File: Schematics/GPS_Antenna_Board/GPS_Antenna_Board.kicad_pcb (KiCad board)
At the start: 2 copper layers, 50 x 65 mm, 28 parts, among them J2 SATA Conn. (Male), U1 SAM-M10Q, U2 LM66100DCKR

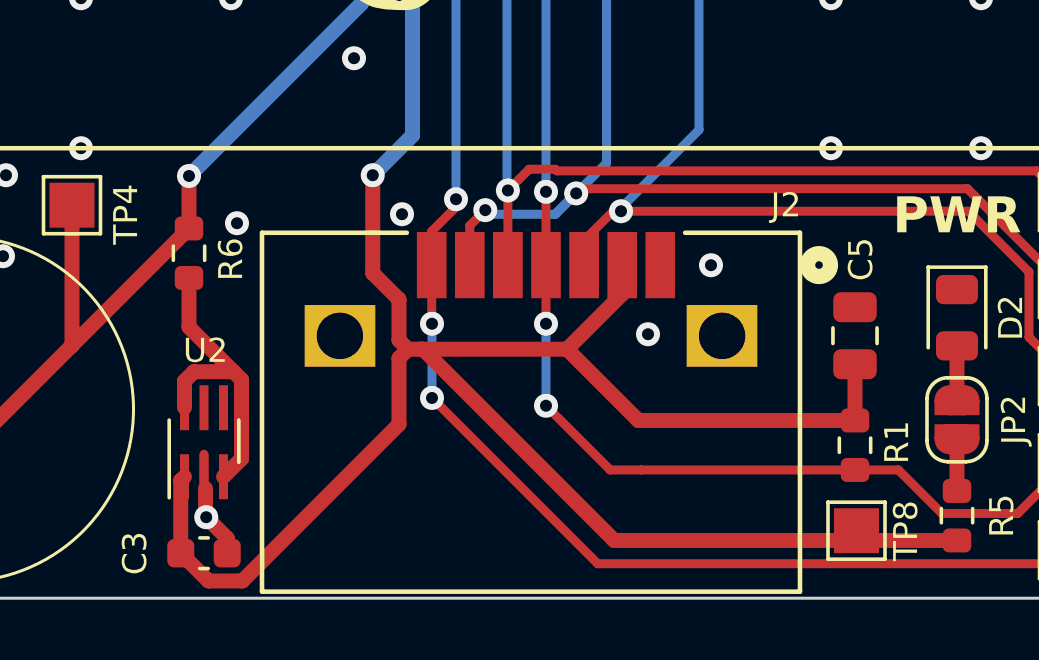
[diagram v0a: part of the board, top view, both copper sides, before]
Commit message: Final Revisions
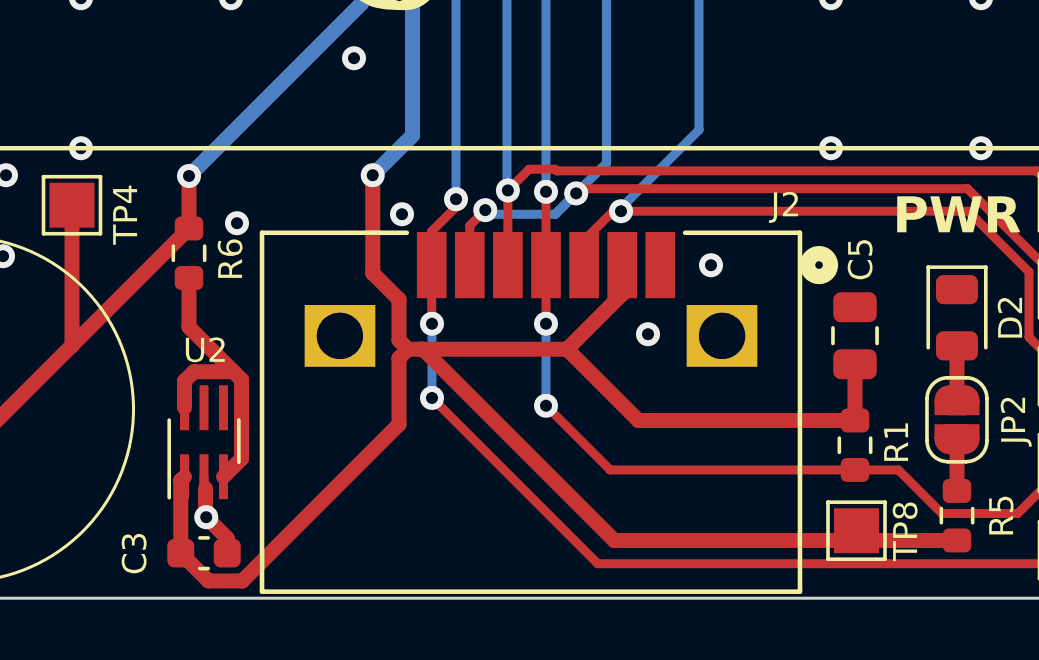
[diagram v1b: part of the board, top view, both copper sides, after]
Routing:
- net GND: track 12.3 -> 11.5 mm
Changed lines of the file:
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@@
     (effects (font (size 1.2 1.2) (thickness 0.2) bold) (justify bottom))
   )
-  (segment (start 136.8 135.15) (end 136.8 134.4) (width 0.3) (layer "F.Cu") (net 1))
   (segment (start 136.85 136.4755) (end 136.85 135.53995) (width 0.5) (layer "F.Cu") (net 1))
   (segment (start 136.8745 136.5) (end 136.85 136.4755) (width 0.5) (layer "F.Cu") (net 1))
@@
   (segment (start 153.3 101.389339) (end 153.3 123.589472) (width 0.3) (layer "B.Cu") (net 6))
   (segment (start 147.010661 95.1) (end 153.3 101.389339) (width 0.3) (layer "B.Cu") (net 6))
-  (segment (start 151.3755 134.925) (end 150.341585 134.925) (width 0.3) (layer "F.Cu") (net 7))
+  (segment (start 150.341585 134.925) (end 158.5 134.925) (width 0.3) (layer "F.Cu") (net 7))
   (segment (start 158.5 134.925) (end 159.947182 134.925) (width 0.3) (layer "F.Cu") (net 7))
   (segment (start 159.947182 134.925) (end 161.397182 136.375) (width 0.3) (layer "F.Cu") (net 7))
@@
   (segment (start 147.7 94.4995) (end 147.7 92) (width 0.3) (layer "F.Cu") (net 7))
   (segment (start 148.2 130.0505) (end 148.199999 128.095301) (width 0.3) (layer "F.Cu") (net 7))
-  (segment (start 151.3755 134.925) (end 158.5 134.925) (width 0.3) (layer "F.Cu") (net 7))
   (segment (start 150.341585 134.925) (end 148.2 132.783415) (width 0.3) (layer "F.Cu") (net 7))
   (segment (start 148.199999 125.6505) (end 148.199999 128.095301) (width 0.3) (layer "F.Cu") (net 7))
@@
   (segment (start 146.929999 125.607571) (end 146.929999 128.095301) (width 0.3) (layer "F.Cu") (net 8))
   (segment (start 147.63707 124.9005) (end 146.929999 125.607571) (width 0.3) (layer "F.Cu") (net 8))
-  (segment (start 146.9 128.1253) (end 146.929999 128.095301) (width 0.5) (layer "F.Cu") (net 8))
   (segment (start 148.56574 124.95558) (end 148.51066 124.9005) (width 0.3) (layer "F.Cu") (net 8))
   (segment (start 149.6 106.4) (end 149.6 104.2) (width 0.3) (layer "F.Cu") (net 8))
@@
   (segment (start 164.55558 124.95558) (end 148.56574 124.95558) (width 0.3) (layer "F.Cu") (net 8))
   (segment (start 148.51066 124.9005) (end 147.63707 124.9005) (width 0.3) (layer "F.Cu") (net 8))
-  (segment (start 146.929999 125.607571) (end 146.929999 125.409339) (width 0.3) (layer "F.Cu") (net 8))
   (via (at 149.6 104.2) (size 0.8) (drill 0.4) (layers "F.Cu" "B.Cu") (net 8))
   (via (at 146.929999 125.607571) (size 0.8) (drill 0.4) (layers "F.Cu" "B.Cu") (net 8))
@@
   (segment (start 148.51066 126.4005) (end 150.219478 124.691682) (width 0.3) (layer "B.Cu") (net 9))
   (segment (start 146.176017 126.263709) (end 146.312808 126.4005) (width 0.3) (layer "B.Cu") (net 9))
-  (segment (start 144.4 128.105302) (end 144.389999 128.095301) (width 0.5) (layer "F.Cu") (net 10))
   (segment (start 144.389999 126.970662) (end 144.389999 128.095301) (width 0.3) (layer "F.Cu") (net 10))
   (segment (start 145.8 106.4) (end 145.8 104.2) (width 0.3) (layer "F.Cu") (net 10))
@@
   (segment (start 144.389999 130.040499) (end 144.4 130.0505) (width 0.3) (layer "F.Cu") (net 10))
   (segment (start 144.389999 128.095301) (end 144.389999 130.040499) (width 0.3) (layer "F.Cu") (net 10))
-  (segment (start 144.4 132.5245) (end 144.4245 132.5245) (width 0.5) (layer "F.Cu") (net 10))
   (segment (start 165.6 137.6) (end 169.275 137.6) (width 0.3) (layer "F.Cu") (net 10))
   (segment (start 144.4 132.5245) (end 149.9255 138.05) (width 0.3) (layer "F.Cu") (net 10))
@@
   (segment (start 169.6 133.9) (end 169.6 135.625) (width 0.5) (layer "F.Cu") (net 11))
   (segment (start 161.9 133.9) (end 161.9 135.625) (width 0.5) (layer "F.Cu") (net 12))
-  (segment (start 136.25 128.575) (end 136.3 128.525) (width 0.5) (layer "F.Cu") (net 13))
   (segment (start 137.786396 131.65) (end 136.463604 131.65) (width 0.5) (layer "F.Cu") (net 13))
   (segment (start 137.786396 131.65) (end 136.3 130.163604) (width 0.5) (layer "F.Cu") (net 13))
